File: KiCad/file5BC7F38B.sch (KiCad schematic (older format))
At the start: 58 parts, among them J301 DB9_Female, P301 ISP/PDI, P302 Thru, P304 Header, SW301 Sync, U301 DS3231, U302 ATmega1284P-AU, U304 SI5351A, U305 74HC1G08, U306 MIC5219-3.3BM5, U307 SN74CB3Q3305, U308 MIC5219-3.3BM5, X301 ASTX-H11-25.MHZ, Y301 20 MHz

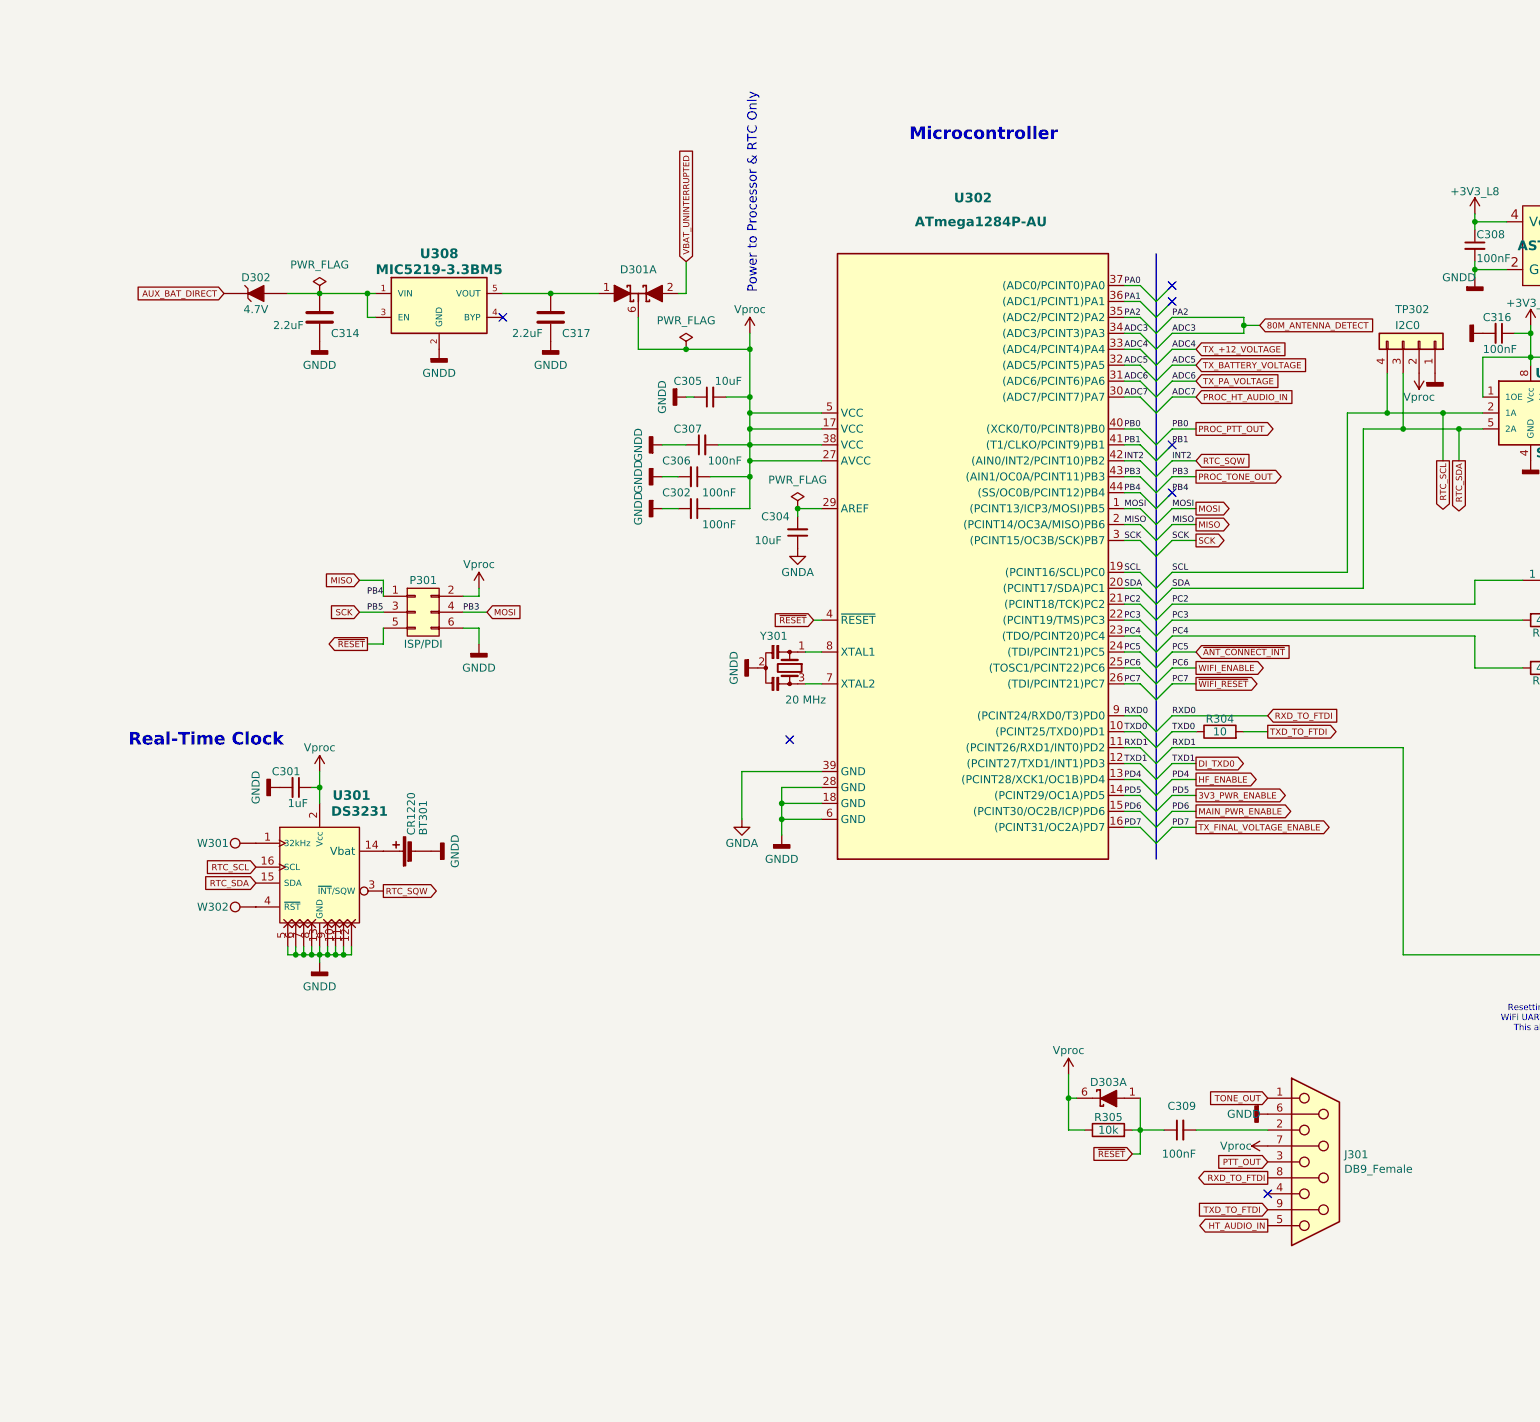
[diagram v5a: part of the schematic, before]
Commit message: Updates to Schematic
Updates to Schematic
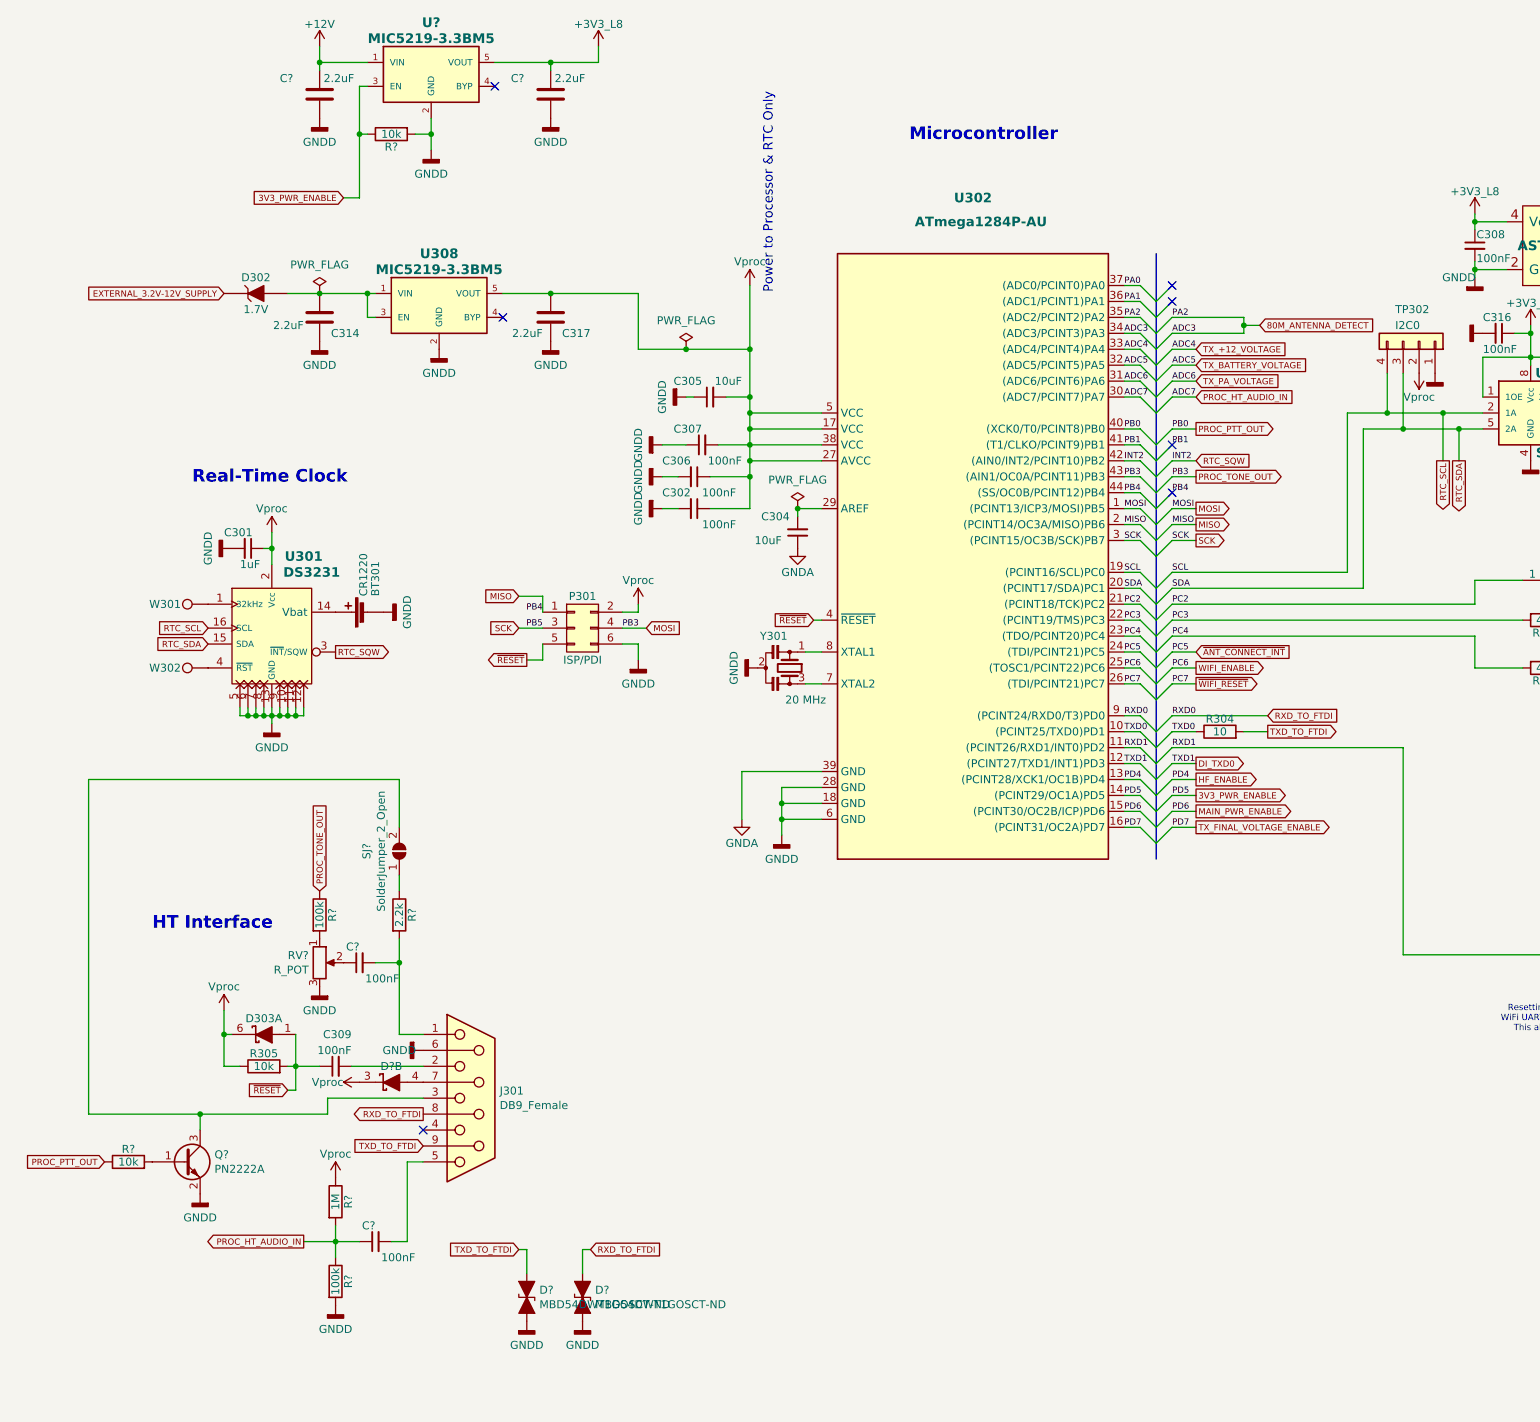
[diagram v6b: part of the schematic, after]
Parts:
- removed D301: D_Schottky_x2_KCom_Dual, TO_SOT_Packages_SMD:SOT-363_Handsolder, symbol FlexFox80-rescue:D_Schottky_x2_KCom_Dual-ARDF-2-Band-MiniTx-rescue
- added C? (x2): 100nF, Capacitors_SMD:C_0805_HandSoldering, symbol Device:C_Small
- added C? (x2): 2.2uF, Capacitors_SMD:C_0805_HandSoldering, symbol Device:C
- added D?: MBD54DWT1GOSCT-ND, TO_SOT_Packages_SMD:SOT-363-0.65, symbol FlexFox80-rescue:MBD54DWT1G_Schottky_Ind-ARDF-2-Band-MiniTx-rescue
- added D? (x2): MBD54DWT1GOSCT-ND, TO_SOT_Packages_SMD:SOT-363-0.65, symbol Diode:ESD9B5.0ST5G
- added Q?: PN2222A, Package_TO_SOT_THT:TO-92_Inline, symbol Transistor_BJT:PN2222A
- added R?: 1M, Resistors_SMD:R_0805_HandSoldering, symbol Device:R
- added R? (x2): 100k, Resistors_SMD:R_0805_HandSoldering, symbol Device:R
- added R? (x2): 10k, Resistors_SMD:R_0805_HandSoldering, symbol Device:R
- added R?: 2.2k, Resistors_SMD:R_0805_HandSoldering, symbol Device:R
- added RV?: R_POT, symbol Device:R_POT
- added SJ?: SolderJumper_2_Open, symbol Jumper:SolderJumper_2_Open
- added U?: MIC5219-3.3BM5, TO_SOT_Packages_SMD:SOT-23-5_Handsolder, symbol FlexFox80-rescue:MIC5219-ARDF-2-Band-MiniTx-rescue
- D302: value 4.7V -> 1.7V
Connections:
- net +12V: now also C?.2, U?.1 (VIN)
- net +3V3_L8: now also C?.2, U?.5 (VOUT)
- net 3V3_PWR_ENABLE: now also R?.1, U?.3 (EN)
- net GND: now also C?.1, C?.1, D?.2 (A2), D?.2 (A2), Q?.2 (E), R?.2, R?.2, RV?.3, U?.2 (GND)
- net MOSI: now also R?.1
- net PROC_HT_AUDIO_IN: now also C?.1, R?.1, R?.2
- net PROC_PTT_OUT: now also R?.1
- net RXD_TO_FTDI: now also D?.1 (A1)
- net TXD_TO_FTDI: now also D?.1 (A1)
- net Vproc: now also C317.2, U308.5 (VOUT), D?.3 (C), R?.1; no longer J301.7
- net AUX_BAT_DIRECT renamed EXTERNAL_3.2V-12V_SUPPLY
- net HT_AUDIO_IN: no longer names the net of J301.5
- net HT_AUDIO_IN: now also C?.2
- net PTT_OUT: no longer names the net of J301.3
- net PTT_OUT: now also Q?.3 (C), SJ?.2 (B)
- net TONE_OUT: no longer names the net of J301.1
- net TONE_OUT: now also C?.2, R?.2
- new net: Q?.1 (B), R?.2
- new net: R?.2, RV?.1
- new net: C?.1, RV?.2
- new net: R?.1, SJ?.1 (A)
- new net: D?.4 (A), J301.7
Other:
- note added: "HT Interface"
- moved on the sheet: BT301, C301, C309, D303A, J301, P301, R305, U301, W301, W302
